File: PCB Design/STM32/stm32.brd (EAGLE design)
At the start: 71.1 x 86.4 mm, 68 parts, among them IC1 NCP1117ST50T3G, Q1 8MHz, T1 SFH303, T2 SFH303, T3 SFH303, T4 SFH303, U1 STM32F103RET6, U2 MCP1700T-3302E/TT, U3 MCP1700T-3302E/TT, U4 MPU-6050, U5 TB6612FNG, X1 22-23-2031

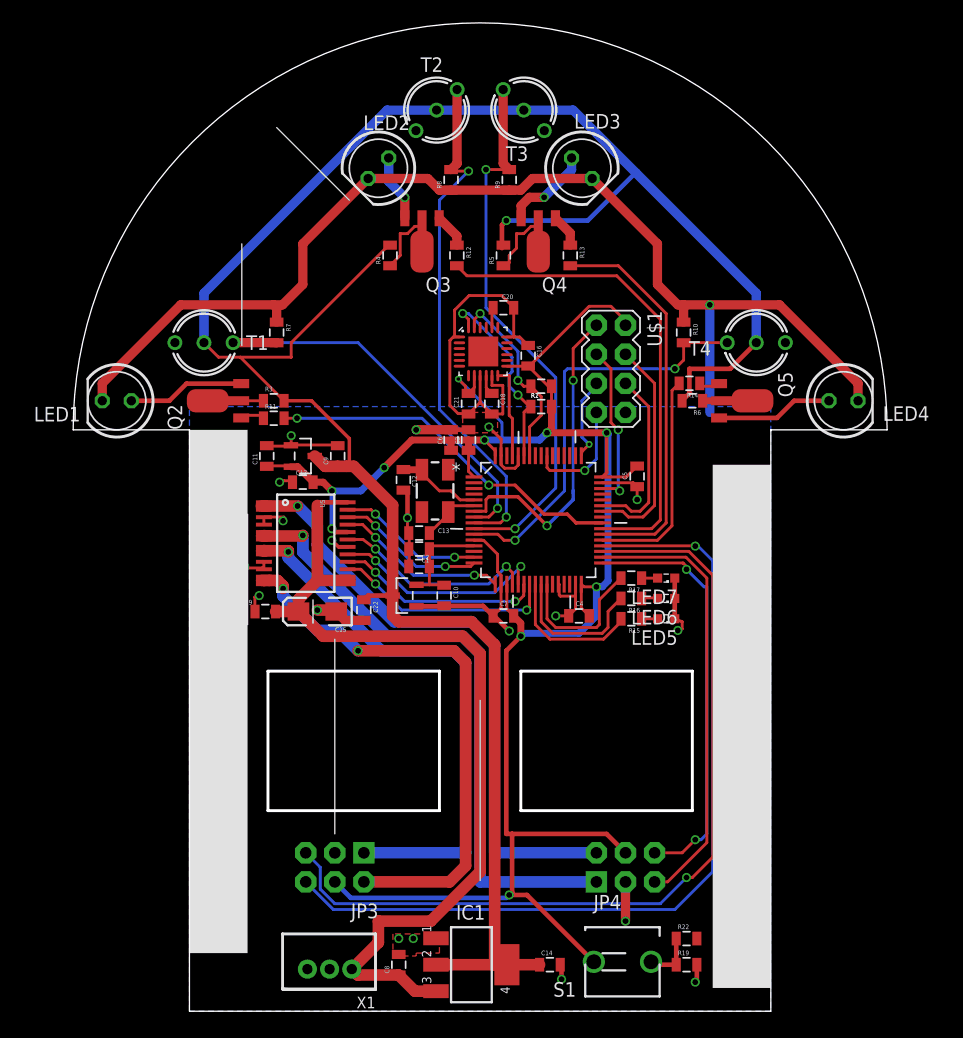
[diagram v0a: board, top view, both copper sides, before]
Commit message: second draft
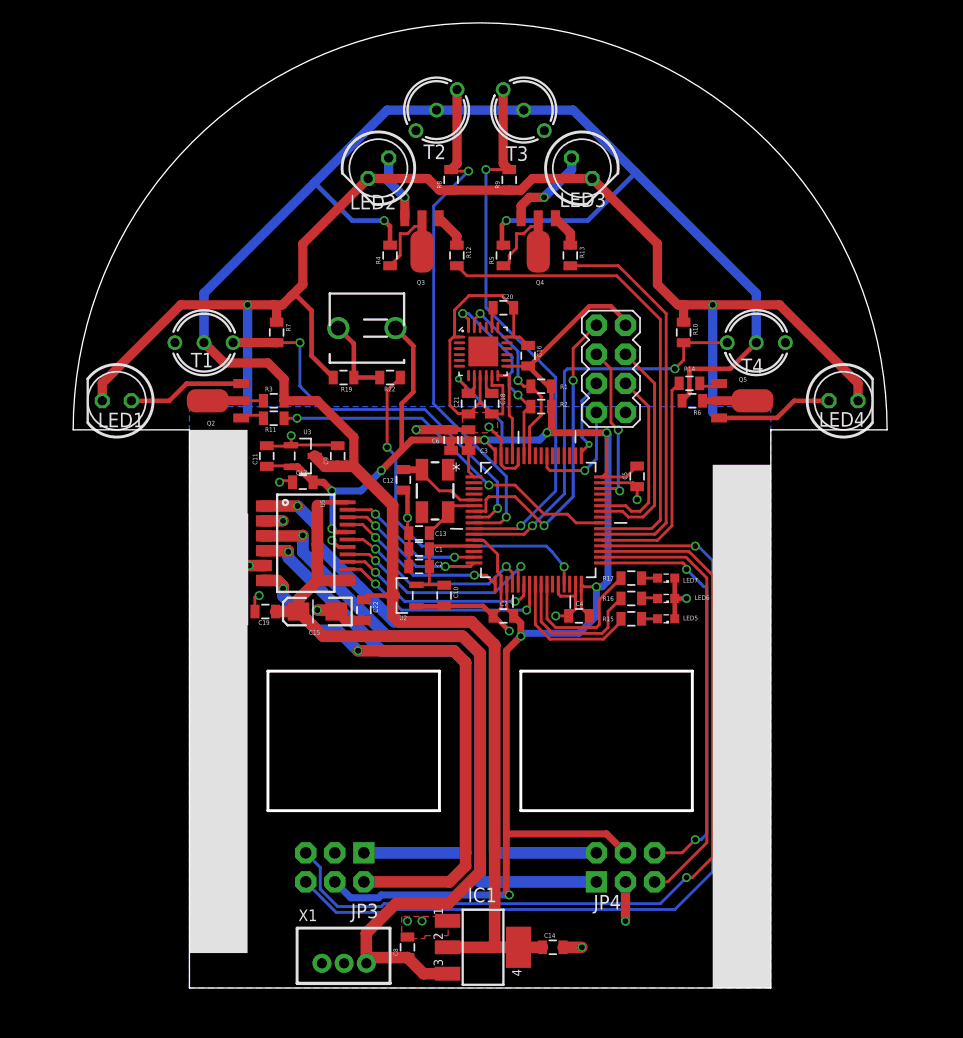
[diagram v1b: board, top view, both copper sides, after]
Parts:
- moved R19 59.4 mm to (74.4, 55.4), turned to 180 degrees
- moved S1 59.2 mm to (77.2, 59.7), turned to 0 degrees
- moved R22 55.4 mm to (78.5, 55.4)
- moved IC1 1.83 mm to (86.6, 5.59)
- moved C8 1.70 mm to (80.0, 5.59)
- moved C14 1.55 mm to (92.7, 5.59)
- moved X1 1.37 mm to (74.7, 5.59)
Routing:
- net BUTTON1: track 0.00 -> 31.2 mm, vias 0 -> 2
- net GND: track 216.1 -> 231.8 mm
- net 5V: track 201.2 -> 192.8 mm, vias 1 -> 2
- net N$31: track 4.59 -> 7.14 mm
- net VCC: track 175.9 -> 177.9 mm
- net IR_IN1: track 36.6 -> 35.1 mm, vias 1 -> 2
- net V_BATT: track 79.0 -> 77.8 mm
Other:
- board size 71.1 x 86.4 mm -> 71.1 x 84.3 mm
